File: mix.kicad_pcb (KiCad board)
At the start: 2 copper layers, 152.1 x 64.7 mm, 65 parts, among them J1 Conn_02x05_Odd_Even, J2 AudioJack2_SwitchT, J3 AudioJack2_SwitchT, J4 AudioJack2_SwitchT, J5 AudioJack2_SwitchT, J6 AudioJack2, Q1 BCM847, Q2 BCM847, U1 TL074, U2 TL072

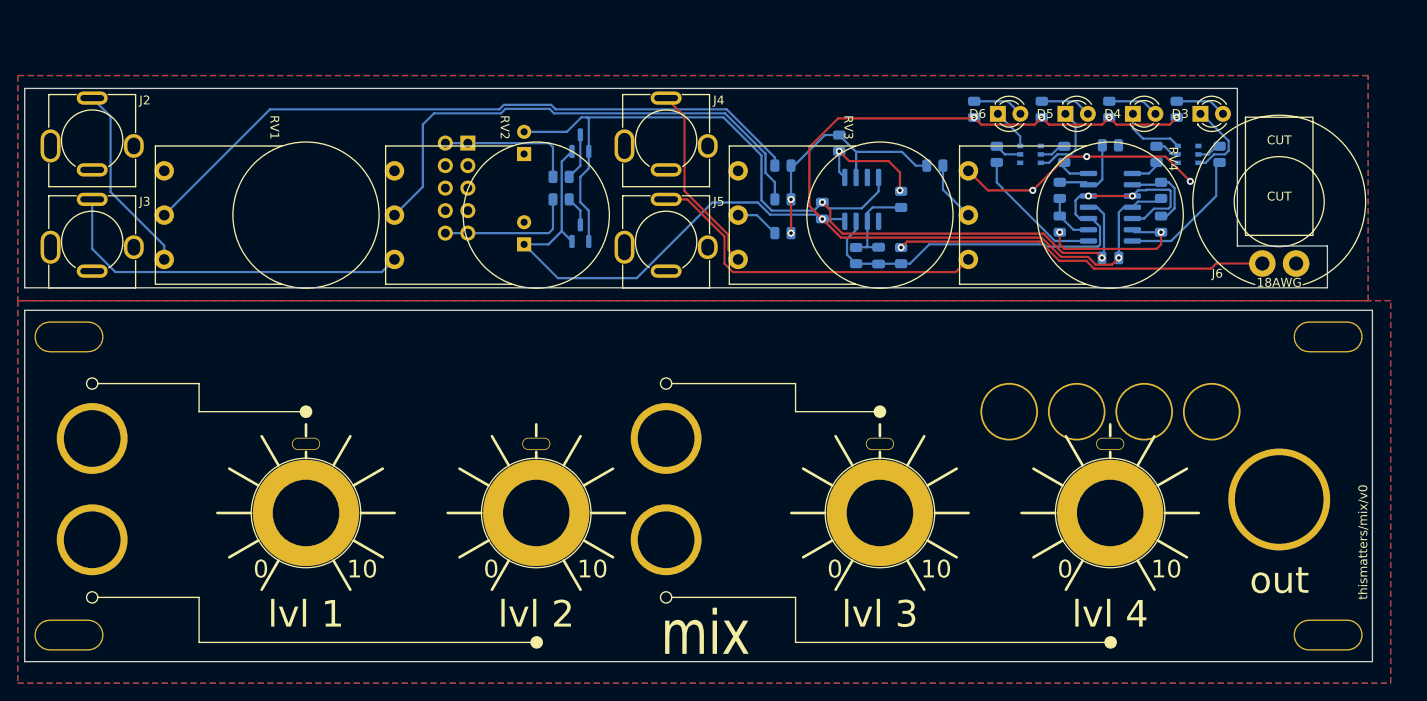
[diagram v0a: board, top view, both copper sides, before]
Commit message: v0
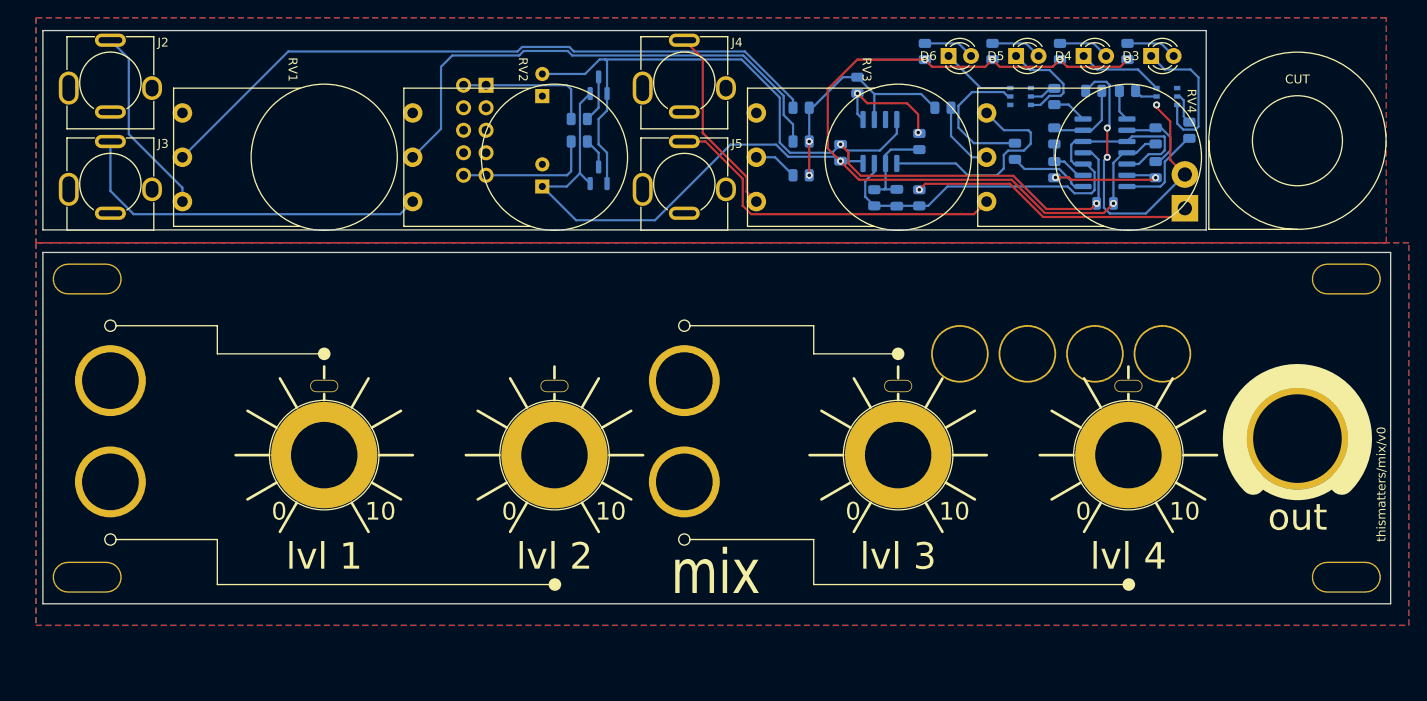
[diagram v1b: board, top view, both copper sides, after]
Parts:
- moved D4 8.58 mm to (170.3, 47.5)
- moved R21 8.58 mm to (167.6, 47.0)
- moved D3 8.58 mm to (177.9, 47.5)
- moved D5 8.58 mm to (162.7, 47.5)
- moved D6 8.58 mm to (155.1, 47.5)
- moved H13 8.58 mm to (179.2, 81.1)
- moved H14 8.58 mm to (171.6, 81.1)
- moved H15 8.58 mm to (164.0, 81.1)
- moved H16 8.58 mm to (156.3, 81.1)
- moved R20 8.58 mm to (175.3, 47.0)
- moved R22 8.58 mm to (160.0, 47.0)
- moved R23 8.58 mm to (152.4, 47.0)
- moved R16 7.88 mm to (175.3, 51.4), turned to 0 degrees
- moved H17 7.17 mm to (194.4, 90.7)
- moved J6 7.17 mm to (194.4, 57.1)
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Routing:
- net GND: track 28.7 -> 63.0 mm
- net Net-(Q2A-B1): track 3.03 -> 16.3 mm
- net /OUT: track 42.5 -> 32.2 mm
- net +12V: track 157.8 -> 148.2 mm
- net Net-(D3-K): track 9.42 -> 16.8 mm
- net Net-(R18-Pad1): track 15.4 -> 9.11 mm
- net Net-(R17-Pad1): track 15.4 -> 10.7 mm
- net Net-(D6-K): track 4.67 -> 8.47 mm
- net Net-(U1B--): track 18.0 -> 15.0 mm
- net Net-(D5-K): track 9.06 -> 11.9 mm
- net /OUT': track 58.7 -> 56.2 mm, vias 2 -> 0
- net Net-(D4-K): track 7.53 -> 9.74 mm
- net -12V: track 107.6 -> 106.0 mm
- net Net-(R6-Pad1): track 6.78 -> 8.20 mm
- net Net-(Q1B-B2): track 2.42 -> 3.65 mm
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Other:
- outline, holes or cut-outs redrawn
- board text added: "S"
- board text added: "T"
